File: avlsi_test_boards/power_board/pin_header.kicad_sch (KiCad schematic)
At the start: 61 parts, among them J5 Conn_02x20_Odd_Even, J6 Conn_02x20_Odd_Even, J7 Conn_02x20_Odd_Even, J8 Conn_02x20_Odd_Even, U11 SN74LVC16T245DLR, U12 SN74LVC16T245DLR, U13 SN74LVC16T245DLR, U14 SN74LVC16T245DLR, U17 SN74LVC16T245DLR, U18 SN74LVC16T245DLR, U19 SN74LVC16T245DLR

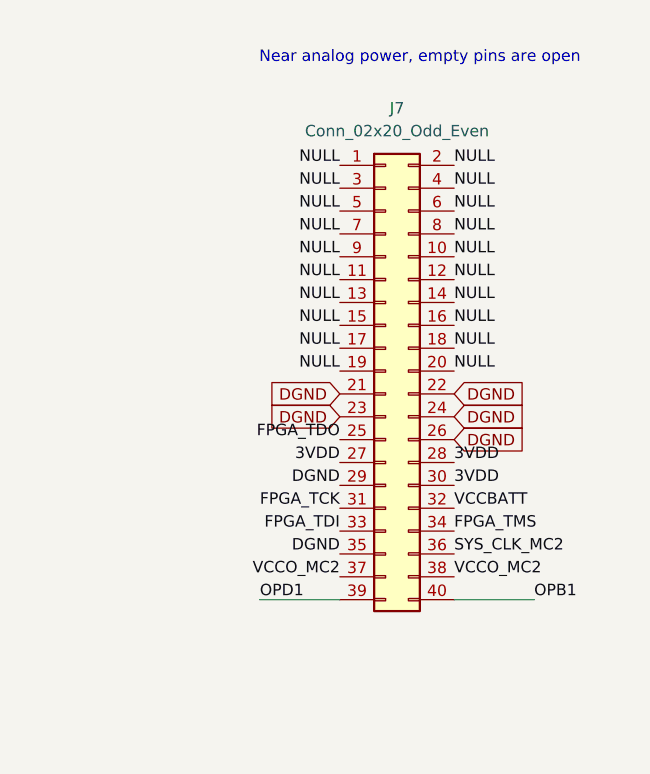
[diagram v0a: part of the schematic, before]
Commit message: more changes
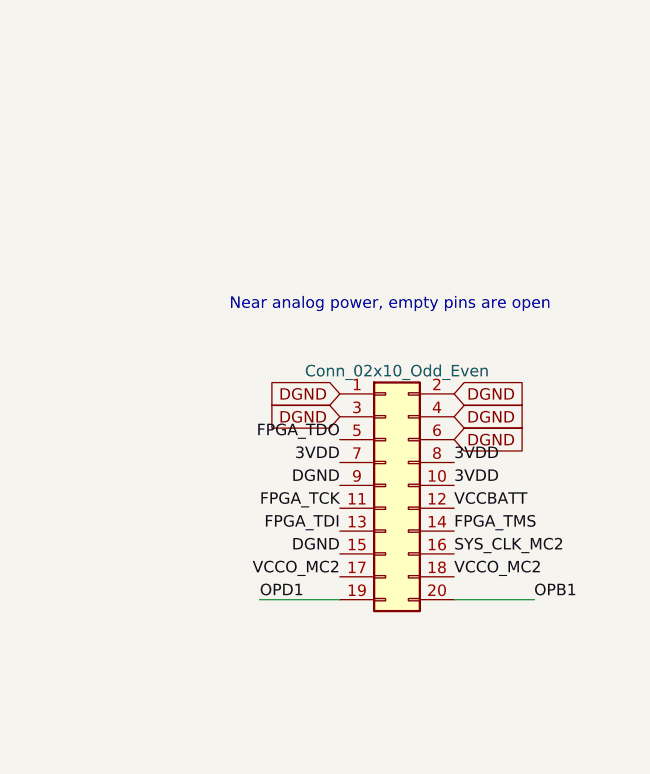
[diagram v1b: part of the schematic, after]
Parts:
- removed J7: Conn_02x20_Odd_Even, Connector_PinHeader_2.00mm:PinHeader_2x20_P2.00mm_Vertical, symbol Connector_Generic:Conn_02x20_Odd_Even
- added J4: Conn_02x10_Odd_Even, Connector_PinHeader_2.00mm:PinHeader_2x10_P2.00mm_Vertical, symbol Connector_Generic:Conn_02x10_Odd_Even
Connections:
- net 3VDD: now also J4.10 (Pin_10), J4.7 (Pin_7), J4.8 (Pin_8)
- net DGND: now also J4.1 (Pin_1), J4.15 (Pin_15), J4.2 (Pin_2), J4.3 (Pin_3), J4.4 (Pin_4), J4.6 (Pin_6), J4.9 (Pin_9)
- net FPGA_TCK: now also J4.11 (Pin_11)
- net FPGA_TDI: now also J4.13 (Pin_13)
- net FPGA_TDO: now also J4.5 (Pin_5)
- net FPGA_TMS: now also J4.14 (Pin_14)
- net OPB1: now also J4.20 (Pin_20)
- net OPD1: now also J4.19 (Pin_19)
- net SYS_CLK_MC2: now also J4.16 (Pin_16)
- net VCCBATT: now also J4.12 (Pin_12)
- net VCCO_MC2: now also J4.17 (Pin_17), J4.18 (Pin_18)
